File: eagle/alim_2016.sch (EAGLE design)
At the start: 54 parts, among them J1 AVR_SPI_PRG_6PTH, J2 AVR_SPI_PRG_6PTH, U1 3.3V, U2 LM2678S-5.0, U4 LM2596S-ADJ, U5 ATTINY85-20SU, U6 ATMEGA328P_TQFP

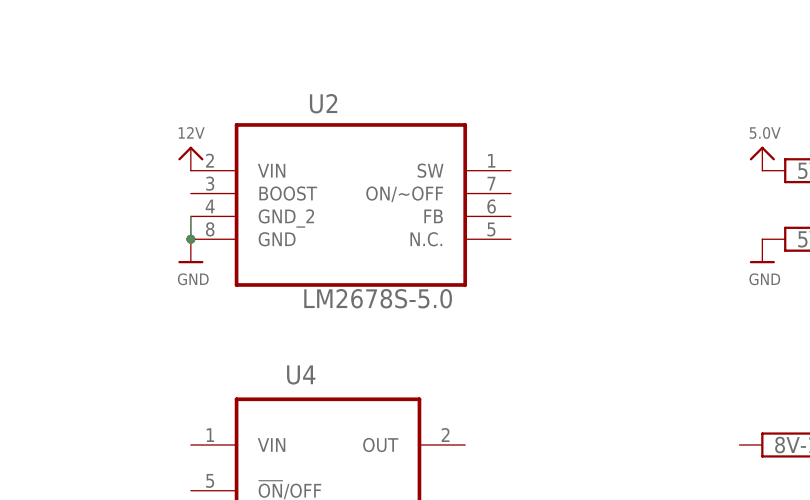
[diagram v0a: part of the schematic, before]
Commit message: clean up board
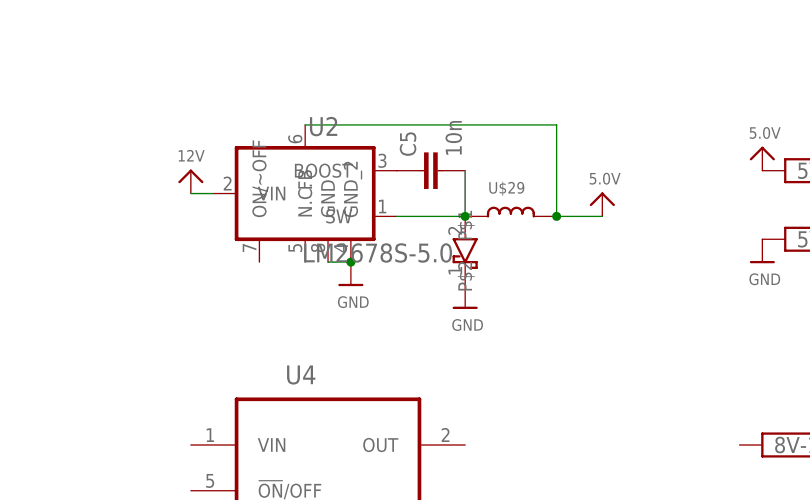
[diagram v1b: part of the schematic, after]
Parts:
- added C5: 10n, rcl:C-EUC0805
- added U$29: SRR1260, alim:SRR1260
- added U$30: SBRS8340, alim:SBRS8340
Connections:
- net N$12 renamed 24V
- new net N$29: C5.2, U$29.1, U$30.P$2, U2.SW
- new net N$30: C5.1, U2.BOOST
- net 5.0V: now also U$29.2, U2.FB
- net GND: now also U$30.P$1
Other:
- moved on the sheet: U2
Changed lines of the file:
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@@
 <layer number="230" name="230bmp" color="7" fill="1" visible="yes" active="yes"/>
 <layer number="231" name="231bmp" color="7" fill="1" visible="yes" active="yes"/>
+<layer number="232" name="Eagle3D_PG2" color="7" fill="1" visible="no" active="no"/>
+<layer number="233" name="Eagle3D_PG3" color="7" fill="1" visible="no" active="no"/>
 <layer number="248" name="Housing" color="7" fill="1" visible="yes" active="yes"/>
 <layer number="249" name="Edge" color="7" fill="1" visible="yes" active="yes"/>
@@
 <part name="R19" library="resistor" deviceset="R-EU_" device="M0805" value="220"/>
 <part name="U$28" library="microbuilder" deviceset="GND" device=""/>
+<part name="U$29" library="alim" deviceset="SRR1260" device=""/>
+<part name="C5" library="rcl" deviceset="C-EU" device="C0805" value="10n"/>
+<part name="U$30" library="alim" deviceset="SBRS8340" device=""/>
+<part name="U$31" library="microbuilder" deviceset="GND" device=""/>
+<part name="U$32" library="microbuilder" deviceset="5.0V" device=""/>
 </parts>
 <sheets>
@@
 <instance part="U$7" gate="G$1" x="124.46" y="-12.7"/>
 <instance part="U2" gate="A" x="106.68" y="55.88"/>
-<instance part="U$22" gate="G$1" x="88.9" y="45.72"/>
+<instance part="U$22" gate="G$1" x="106.68" y="43.18"/>
 <instance part="U4" gate="A" x="104.14" y="22.86"/>
 <instance part="U$23" gate="G$1" x="88.9" y="10.16"/>
@@
 <instance part="R5" gate="G$1" x="-27.94" y="30.48" rot="R180"/>
 <instance part="S1" gate="G$1" x="-22.86" y="38.1" rot="MR90"/>
-<instance part="U$4" gate="G$1" x="88.9" y="58.42"/>
+<instance part="U$4" gate="G$1" x="88.9" y="55.88"/>
 <instance part="12V" gate="-1" x="-2.54" y="43.18"/>
 <instance part="12V" gate="-2" x="-2.54" y="22.86"/>
@@
 <instance part="R19" gate="G$1" x="142.24" y="-91.44" rot="R180"/>
 <instance part="U$28" gate="G$1" x="147.32" y="-99.06"/>
+<instance part="U$29" gate="G$1" x="124.46" y="50.8"/>
+<instance part="C5" gate="G$1" x="114.3" y="55.88" rot="R90"/>
+<instance part="U$30" gate="G$1" x="119.38" y="45.72" rot="R270"/>
+<instance part="U$31" gate="G$1" x="119.38" y="40.64"/>
+<instance part="U$32" gate="G$1" x="134.62" y="53.34"/>
 </instances>
 <busses>
@@
 <pinref part="U$22" gate="G$1" pin="GND"/>
 <pinref part="U2" gate="A" pin="GND_2"/>
-<wire x1="88.9" y1="50.8" x2="88.9" y2="48.26" width="0.1524" layer="91"/>
-<junction x="88.9" y="48.26"/>
+<junction x="106.68" y="45.72"/>
+<wire x1="106.68" y1="45.72" x2="104.14" y2="45.72" width="0.1524" layer="91"/>
 </segment>
 <segment>
@@
 <pinref part="U$28" gate="G$1" pin="GND"/>
 </segment>
+<segment>
+<pinref part="U$30" gate="G$1" pin="P$1"/>
+<pinref part="U$31" gate="G$1" pin="GND"/>
+</segment>
 </net>
 <net name="5.0V" class="0">
@@
 <pinref part="5V" gate="-1" pin="K"/>
 <pinref part="U$3" gate="G$1" pin="5.0V"/>
+</segment>
+<segment>
+<pinref part="U2" gate="A" pin="FB"/>
+<wire x1="101.6" y1="60.96" x2="129.54" y2="60.96" width="0.1524" layer="91"/>
+<pinref part="U$29" gate="G$1" pin="2"/>
+<wire x1="129.54" y1="60.96" x2="129.54" y2="50.8" width="0.1524" layer="91"/>
+<pinref part="U$32" gate="G$1" pin="5.0V"/>
+<wire x1="129.54" y1="50.8" x2="134.62" y2="50.8" width="0.1524" layer="91"/>
+<junction x="129.54" y="50.8"/>
 </segment>
 </net>
@@
 </segment>
 </net>
-<net name="N$12" class="0">
+<net name="24V" class="0">
 <segment>
 <pinref part="BAT2" gate="-1" pin="KL"/>
@@
 <pinref part="U2" gate="A" pin="VIN"/>
 <pinref part="U$4" gate="G$1" pin="12V"/>
+<wire x1="88.9" y1="53.34" x2="91.44" y2="53.34" width="0.1524" layer="91"/>
 </segment>
 </net>
@@
 </segment>
 </net>
+<net name="N$29" class="0">
+<segment>
+<pinref part="U2" gate="A" pin="SW"/>
+<pinref part="U$29" gate="G$1" pin="1"/>
+<pinref part="C5" gate="G$1" pin="2"/>
+<wire x1="119.38" y1="55.88" x2="119.38" y2="50.8" width="0.1524" layer="91"/>
+<junction x="119.38" y="50.8"/>
+<wire x1="119.38" y1="50.8" x2="111.76" y2="50.8" width="0.1524" layer="91"/>
+<pinref part="U$30" gate="G$1" pin="P$2"/>
+</segment>
+</net>
+<net name="N$30" class="0">
+<segment>
+<pinref part="U2" gate="A" pin="BOOST"/>
+<pinref part="C5" gate="G$1" pin="1"/>
+</segment>
+</net>

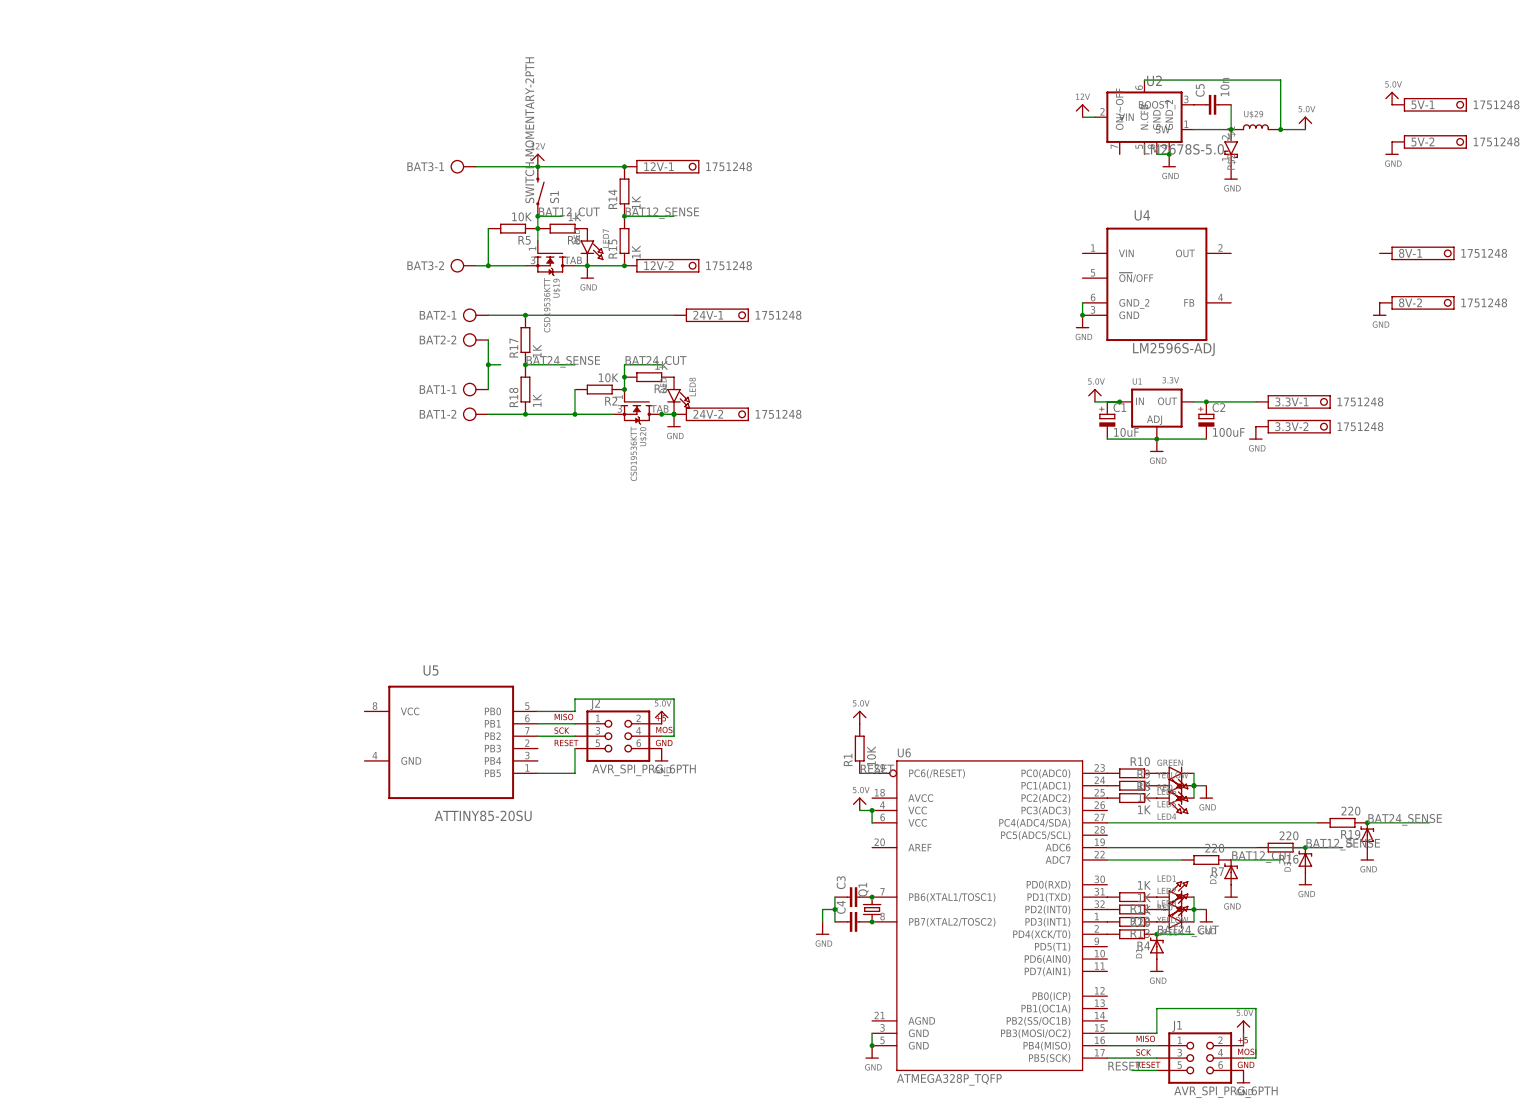
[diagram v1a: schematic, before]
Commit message: most of the circuit finished
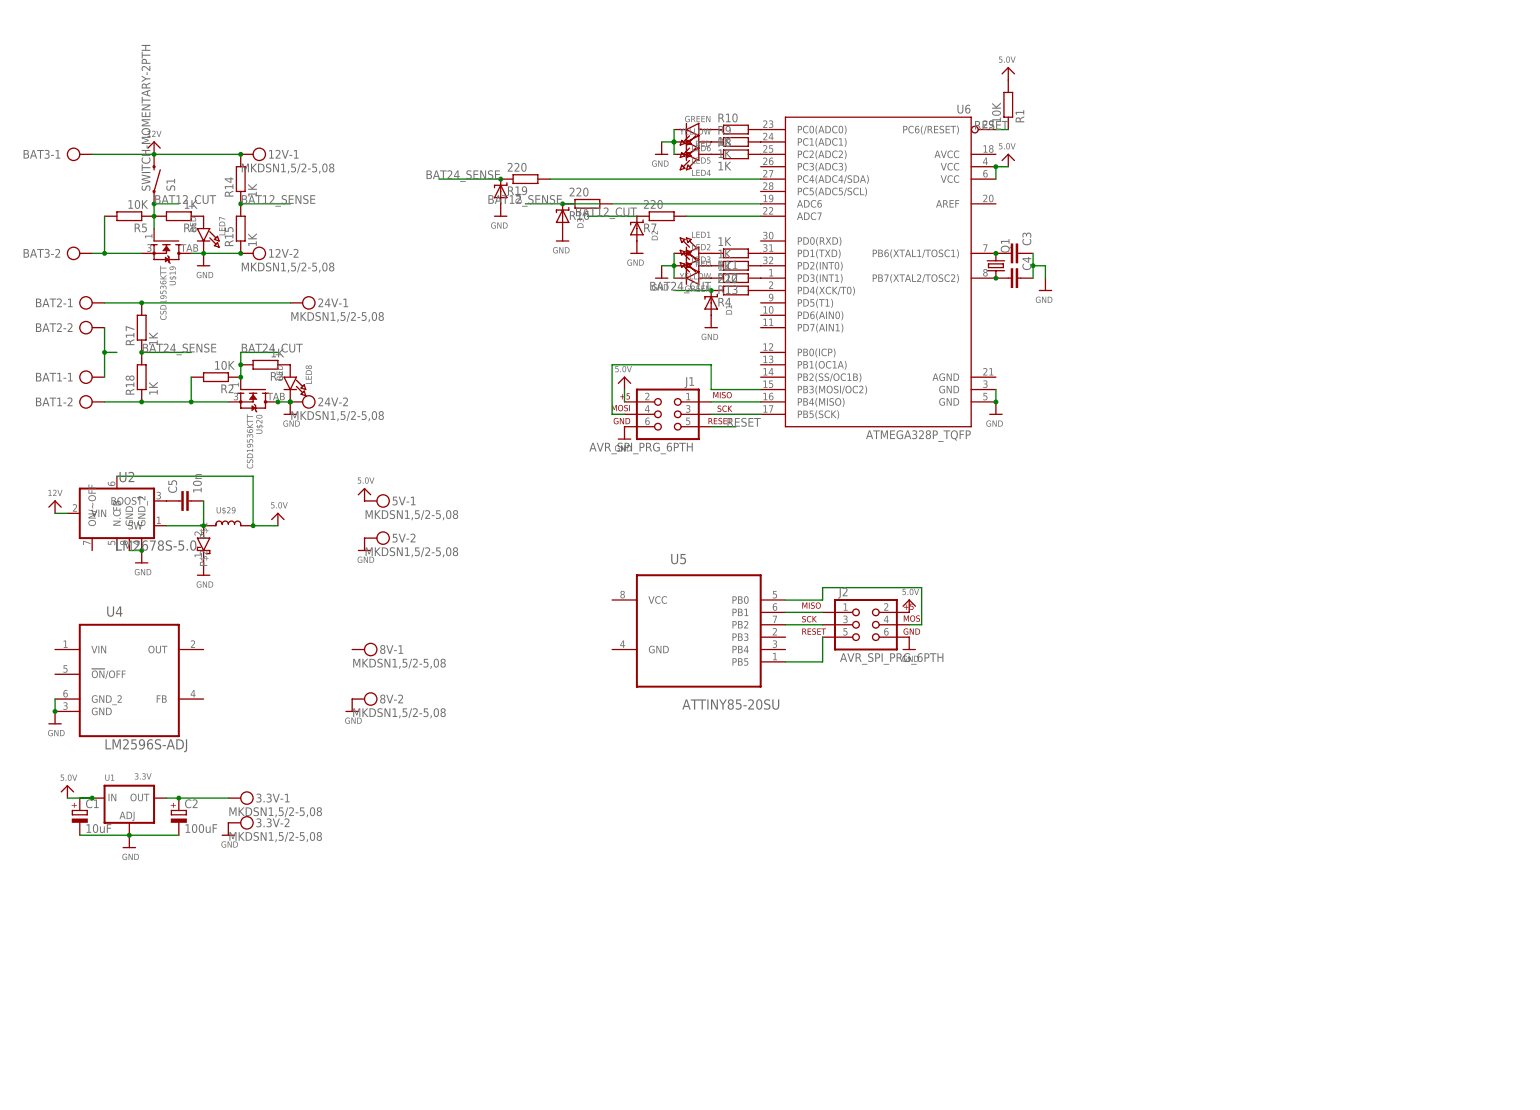
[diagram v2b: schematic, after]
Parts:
- 12V, 24V, 3.3V, 5V, 8V: value 1751248 -> MKDSN1,5/2-5,08; device con-phoenix-350:1751248 -> con-phoenix-508:MKDSN1,5/2-5,08
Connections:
- net 12V: now also 12V-1.KL; no longer 12V-1.K
- net 24V: now also 24V-1.KL; no longer 24V-1.K
- net 5.0V: now also 5V-1.KL; no longer 5V-1.K
- net GND: now also 12V-2.KL, 24V-2.KL, 3.3V-2.KL, 5V-2.KL, 8V-2.KL; no longer 12V-2.K, 24V-2.K, 3.3V-2.K, 5V-2.K, 8V-2.K
- net N$1: now also 3.3V-1.KL; no longer 3.3V-1.K
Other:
- moved on the sheet: BAT1-1, BAT1-2, BAT2-1, BAT2-2, BAT3-1, BAT3-2, C1, C2, C3, C4, C5, D1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

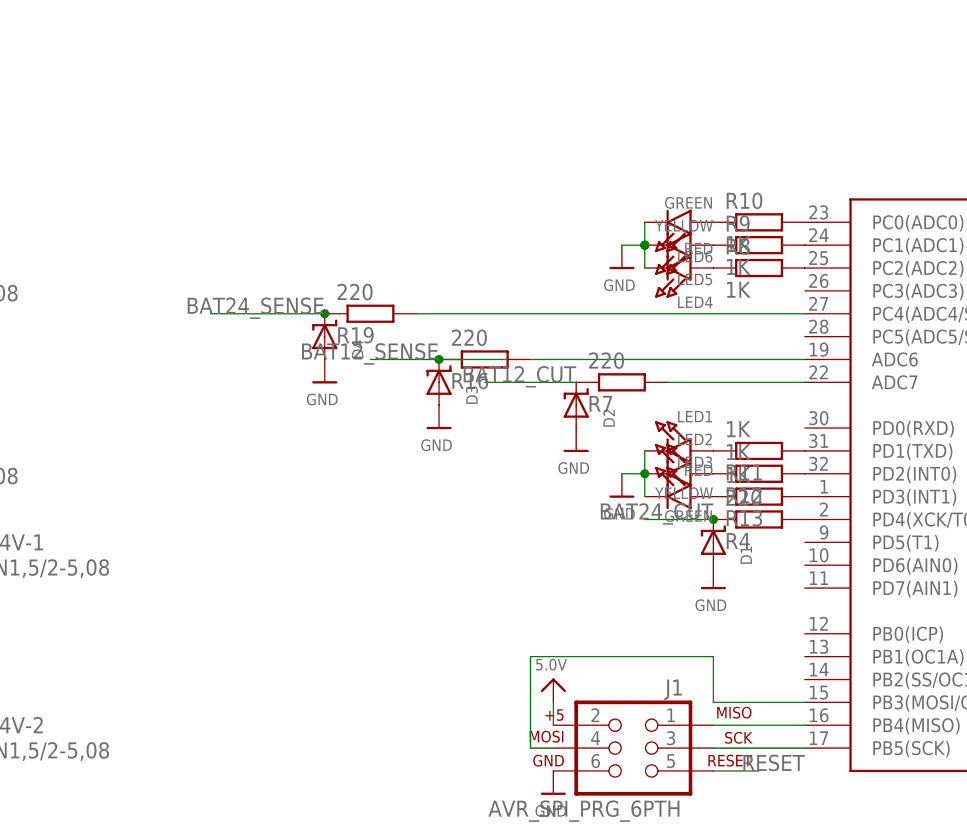
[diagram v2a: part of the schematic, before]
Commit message: more cleanup
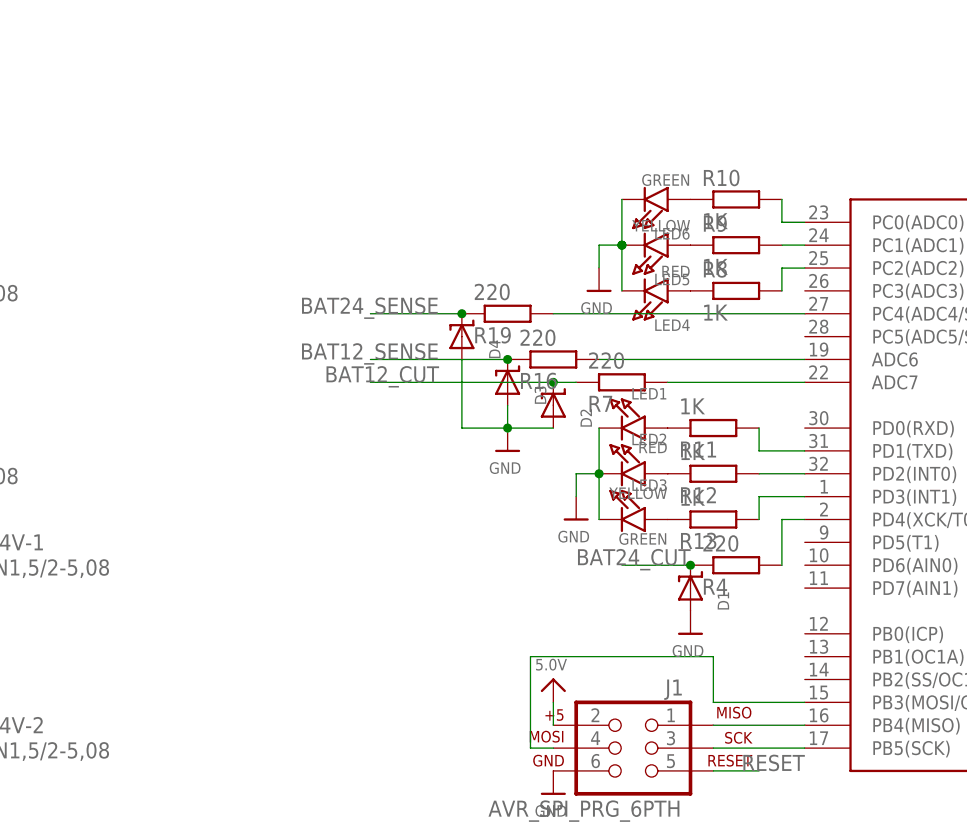
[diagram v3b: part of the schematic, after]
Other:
- moved on the sheet: D1, D2, D3, D4, LED1, LED2, LED3, LED4, LED5, LED6, R10, R11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

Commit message: rearrange stuff
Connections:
- net N$29 renamed SW
- net N$30 renamed BOOST
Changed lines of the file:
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@@
 </segment>
 </net>
-<net name="N$29" class="0">
+<net name="SW" class="0">
 <segment>
 <pinref part="U2" gate="A" pin="SW"/>
@@
 </segment>
 </net>
-<net name="N$30" class="0">
+<net name="BOOST" class="0">
 <segment>
 <pinref part="U2" gate="A" pin="BOOST"/>
